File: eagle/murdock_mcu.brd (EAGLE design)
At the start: 47 x 31.8 mm, 17 parts, among them IC1 MPU-6050, IC2 LT1763CS8-3.3, U1 USD-SOCKETNEW, X1 USBSMD, X2 MURDOCK_STACK

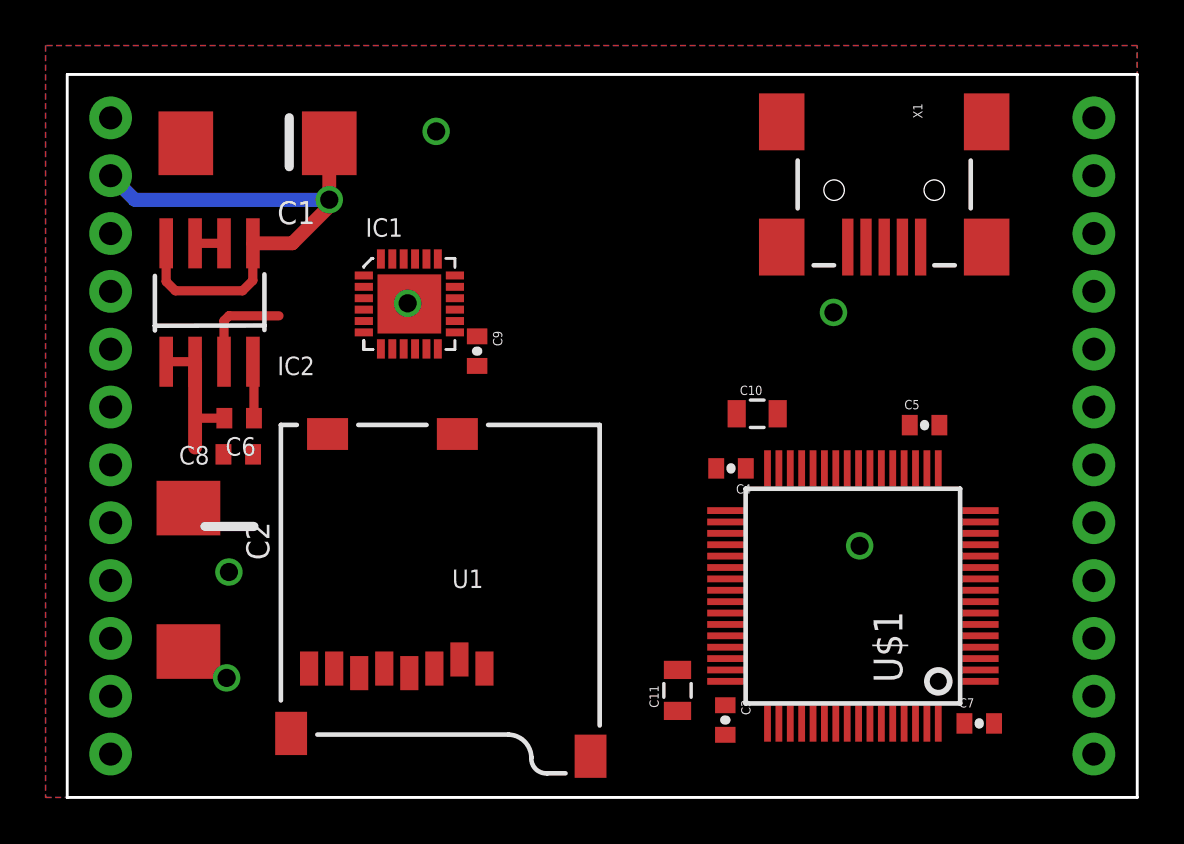
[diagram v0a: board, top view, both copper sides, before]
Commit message: power and pwm routing
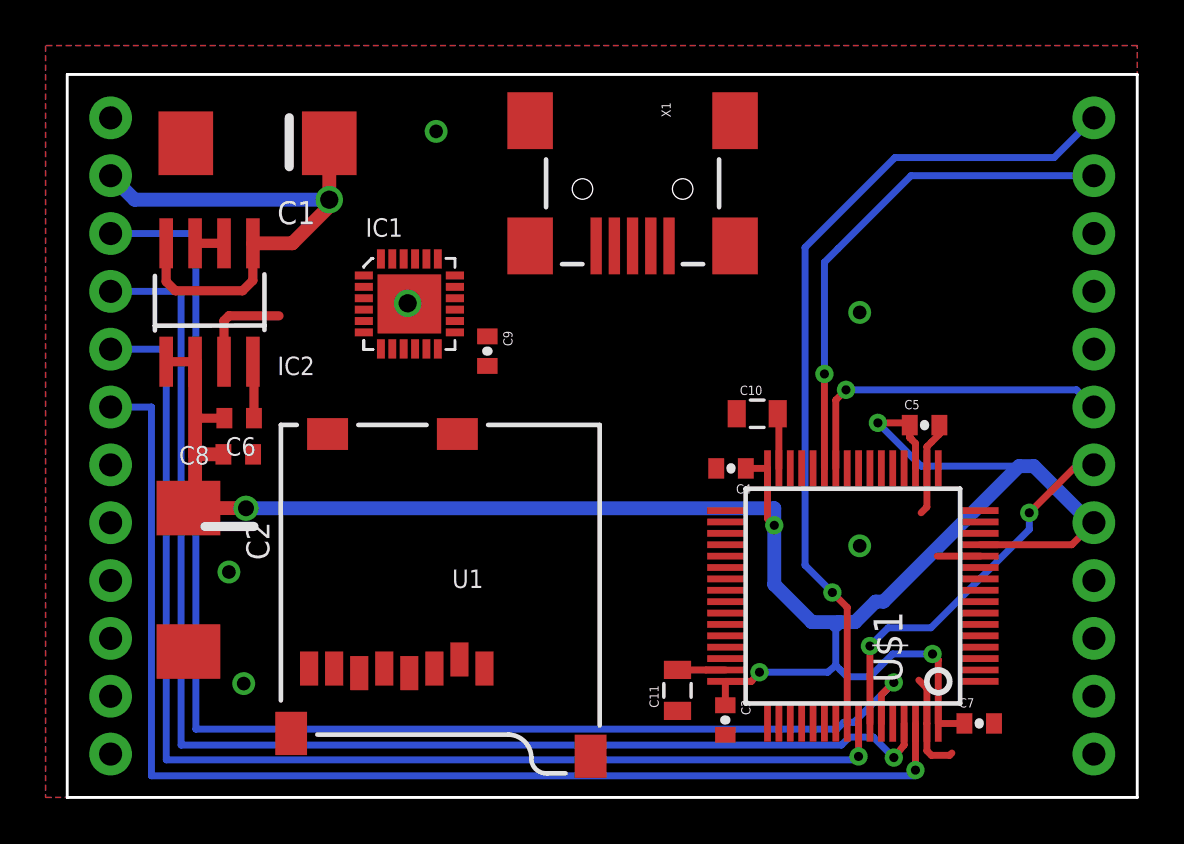
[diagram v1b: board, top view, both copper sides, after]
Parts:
- moved X1 11.1 mm to (24.8, 26.7)
- moved C9 0.45 mm to (18.4, 19.6)
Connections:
- new net PPM: U$1.58, X2.PPM
- new net PWM1: U$1.59, X2.PWM1
- new net PWM2: U$1.61, X2.PWM2
- new net PWM3: U$1.62, X2.PWM3
- new net PWM4: U$1.57, X2.PWM4
- new net PWM5: U$1.56, X2.PWM5
- new net PWM6: U$1.27, X2.PWM6
- new net PWM7: U$1.26, X2.PWM7
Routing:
- net +3V3: track 8.88 -> 97.7 mm, vias 0 -> 5
- net PWM1: track 0.00 -> 59.0 mm, vias 0 -> 1
- net PWM2: track 0.00 -> 56.5 mm, vias 0 -> 1
- net PWM3: track 0.00 -> 53.8 mm, vias 0 -> 1
- net PWM4: track 0.00 -> 52.5 mm, vias 0 -> 1
- net PWM5: track 0.00 -> 36.7 mm, vias 0 -> 1
- net PWM6: track 0.00 -> 22.5 mm, vias 0 -> 1
- net PPM: track 0.00 -> 17.0 mm, vias 0 -> 2
- net PWM7: track 0.00 -> 14.8 mm, vias 0 -> 1
- net GND: track 5.57 -> 16.1 mm
- net N$3: track 0.00 -> 2.42 mm
- net N$4: track 0.00 -> 2.10 mm

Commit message: more routing
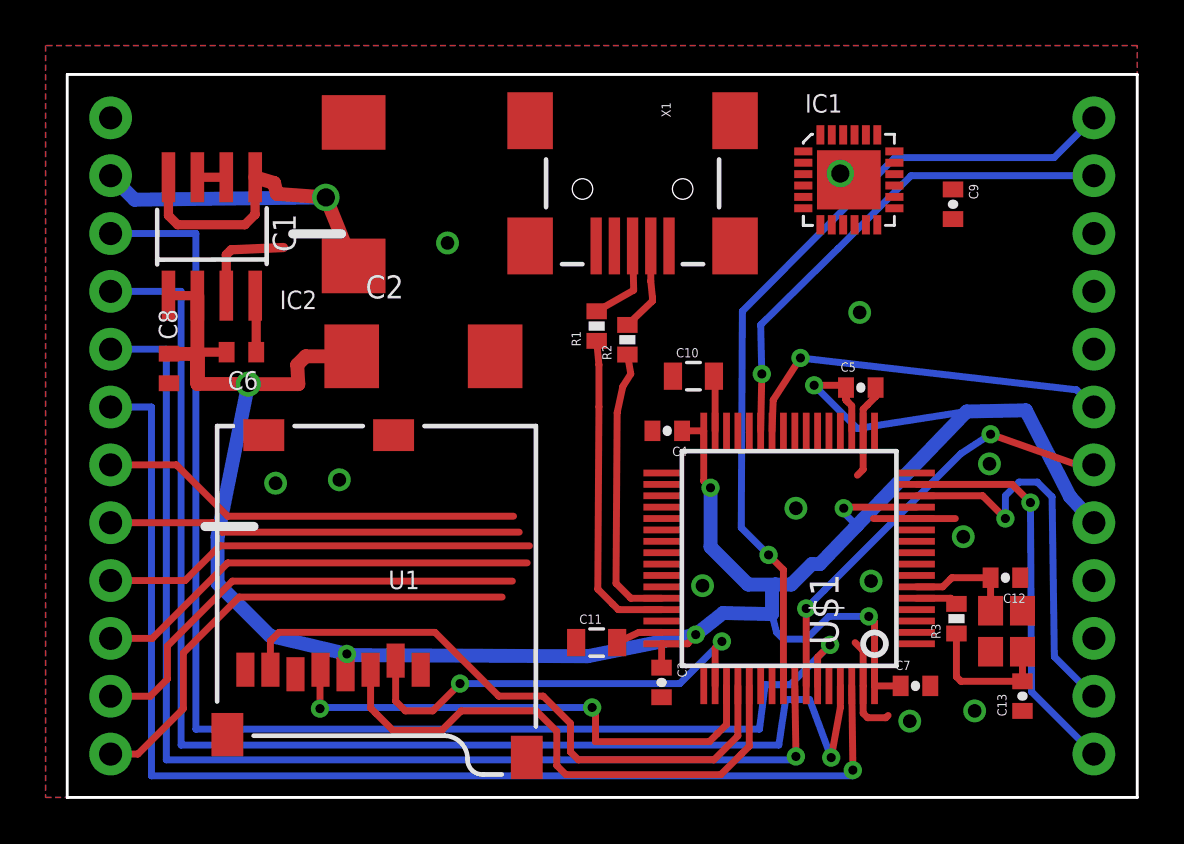
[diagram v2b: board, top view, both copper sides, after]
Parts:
- added C12, C13: (no value), SparkFun-Capacitors:0402-CAP
- added L1: (no value), seb:X22
- added R1, R2, R3: (no value), SparkFun-Resistors:0402-RES
- moved C9 21.4 mm to (38.9, 26.1)
- moved IC1 20.1 mm to (34.3, 27.1)
- moved C2 14.2 mm to (15.6, 19.4), turned to 0 degrees
- moved C8 4.85 mm to (4.47, 18.8), turned to 90 degrees
- moved C1 4.78 mm to (12.6, 26.5), turned to 90 degrees
- moved C11 4.12 mm to (23.2, 6.80), turned to 0 degrees
- moved C10 3.25 mm to (27.5, 18.5)
- moved C4 3.25 mm to (26.4, 16.1)
- moved C3 3.25 mm to (26.1, 5.05)
- moved C7 3.25 mm to (37.2, 4.90)
- moved U$1 3.25 mm to (31.7, 10.5)
- moved C5 3.25 mm to (34.9, 18.0)
- moved IC2 2.90 mm to (6.35, 24.6)
- moved C6 2.90 mm to (7.65, 19.6)
- moved U1 2.80 mm to (6.58, 16.3)
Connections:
- new net A10: U$1.43, X2.SP1
- new net A11: R2.1, U$1.44
- new net A12: R1.1, U$1.45
- new net C7: U$1.38, X2.SP2
- new net MISO: U$1.52, U1.7
- new net MOSI: U$1.53, U1.3
- new net N$1: R2.2, X1.D-
- new net N$2: R1.2, X1.D+
- new net N$5: R3.2, U$1.5
- new net N$6: C13.2, L1.1, R3.1
- new net N$7: C12.2, L1.3, U$1.6
- new net N$8: X2.3V3_SP, X2.SW1
- new net N$9: X2.SW2, X2.SW3
- new net RX: U$1.15, X2.RX
- new net SCK: U$1.51, U1.5
- new net SD_CS: U$1.50, U1.2
- new net TX: U$1.14, X2.TX
- net GND: now also C12.1, C13.1
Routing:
- net N$8: track 0.00 -> 42.1 mm
- net N$9: track 0.00 -> 36.7 mm
- net MISO: track 0.00 -> 27.6 mm
- net MOSI: track 0.00 -> 24.3 mm
- net SCK: track 0.00 -> 23.0 mm, vias 0 -> 2
- net A10: track 0.00 -> 19.7 mm
- net SD_CS: track 0.00 -> 19.6 mm, vias 0 -> 2
- net C7: track 0.00 -> 19.0 mm
- net +3V3: track 97.7 -> 115.6 mm, vias 5 -> 7
- net RX: track 0.00 -> 17.5 mm, vias 0 -> 1
- net TX: track 0.00 -> 17.4 mm, vias 0 -> 1
- net A12: track 0.00 -> 14.1 mm
- net A11: track 0.00 -> 12.5 mm
- net N$6: track 0.00 -> 6.18 mm
- net N$7: track 0.00 -> 4.86 mm
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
